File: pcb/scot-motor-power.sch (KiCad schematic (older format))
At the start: 1 part

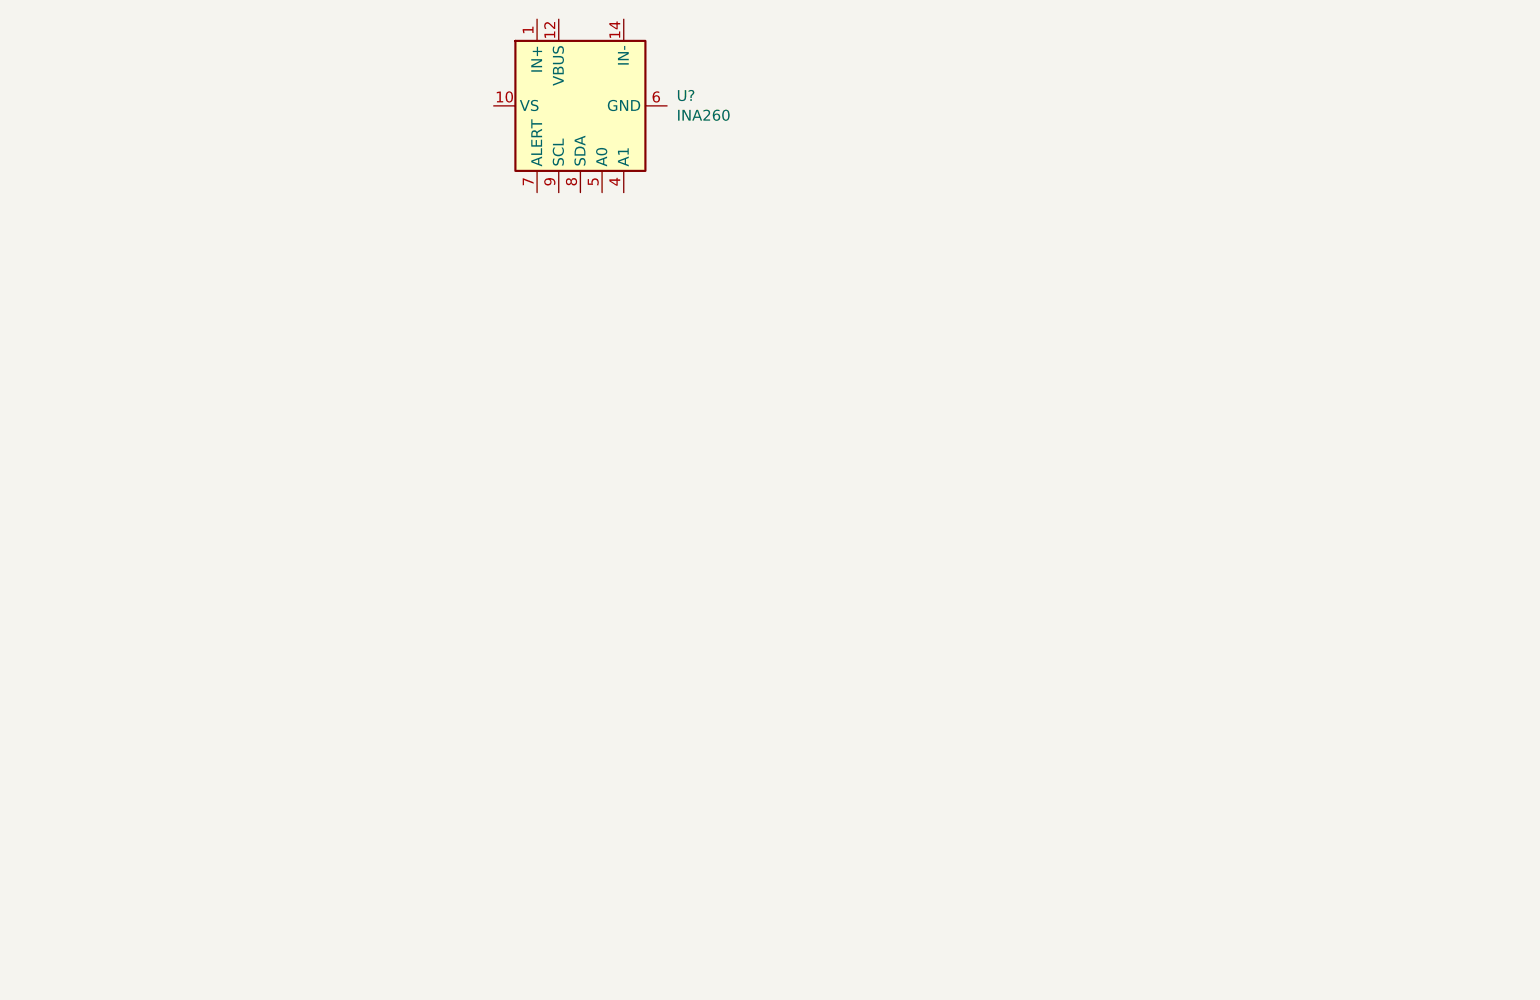
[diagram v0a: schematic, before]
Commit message: WIP.
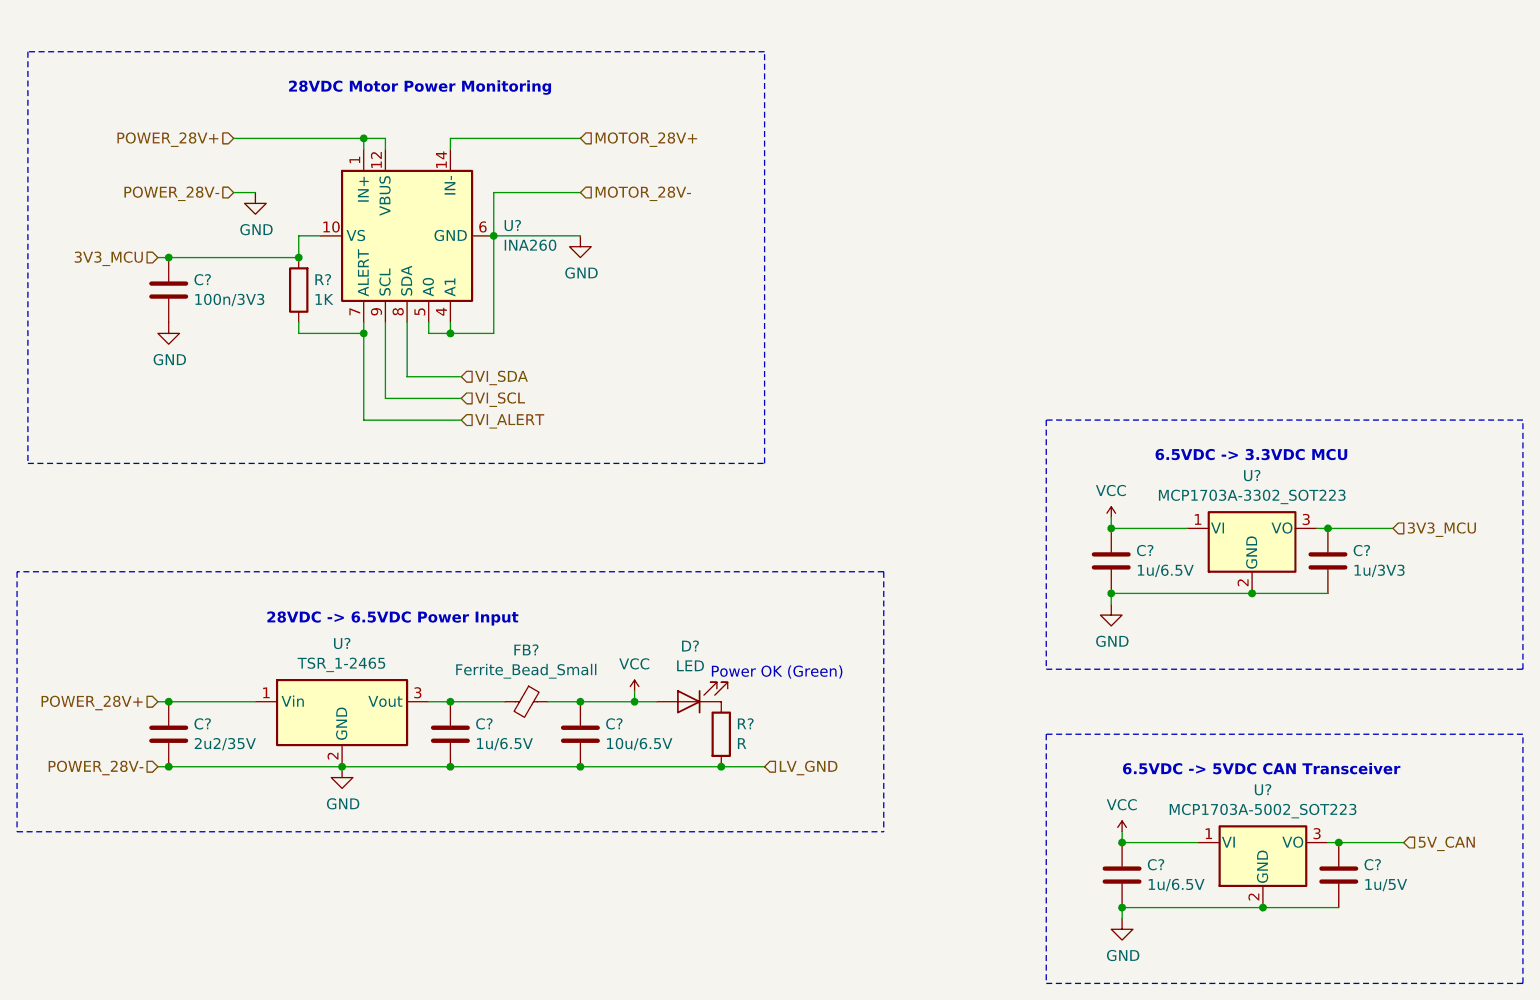
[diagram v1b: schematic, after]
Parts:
- added C?: 2u2/35V, symbol Device:C
- added C? (x3): 1u/6.5V, symbol Device:C
- added C?: 10u/6.5V, symbol Device:C
- added C?: 1u/3V3, symbol Device:C
- added C?: 1u/5V, symbol Device:C
- added C?: 100n/3V3, symbol Device:C
- added D?: LED, symbol Device:LED
- added FB?: Ferrite_Bead_Small, symbol Device:Ferrite_Bead_Small
- added R?: 1K, symbol Device:R
- added R?: R, symbol Device:R
- added U?: MCP1703A-3302_SOT223, Package_TO_SOT_SMD:SOT-223-3_TabPin2, symbol Regulator_Linear:MCP1703A-3302_SOT223
- added U?: MCP1703A-5002_SOT223, Package_TO_SOT_SMD:SOT-223-3_TabPin2, symbol Regulator_Linear:MCP1703A-5002_SOT223
- added U?: TSR_1-2465, Converter_DCDC:Converter_DCDC_TRACO_TSR-1_THT, symbol Regulator_Switching:TSR_1-2465
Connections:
- net POWER_28V+: now reaches U?.1 (IN+), U?.2 (IN+), U?.3 (IN+)
- net POWER_28V+: now also U?.12 (VBUS), C?.1, U?.1 (Vin)
- net 3V3_MCU: now reaches U?.10 (VS)
- net 3V3_MCU: now also C?.1, C?.1, R?.2, U?.3 (VO)
- net GND: now reaches U?.11 (GND), U?.6 (GND)
- net GND: now also U?.4 (A1), U?.5 (A0), C?.2, C?.2, C?.2, C?.2, C?.2, C?.2, C?.2, C?.2, R?.2, U?.2 (GND), U?.2 (GND), U?.2 (GND)
- net MOTOR_28V+: now reaches U?.14 (IN-), U?.15 (IN-), U?.16 (IN-)
- net VI_ALERT: now reaches U?.7 (ALERT)
- net VI_ALERT: now also R?.1
- net VI_SDA: now reaches U?.8 (SDA)
- net VI_SCL: now reaches U?.9 (SCL)
- new net: C?.1, FB?.2, U?.3 (Vout)
- new net: D?.1 (K), R?.1
- new net 5V_CAN: C?.1, U?.3 (VO)
- new net VCC: C?.1, C?.1, C?.1, D?.2 (A), FB?.1, U?.1 (VI), U?.1 (VI)
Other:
- note added: "28VDC -> 6.5VDC Power Input"
- note added: "28VDC Motor Power Monitoring"
- note added: "6.5VDC -> 3.3VDC MCU"
- note added: "6.5VDC -> 5VDC CAN Transceiver"
- note added: "Power OK (Green)"
- moved on the sheet: U?
